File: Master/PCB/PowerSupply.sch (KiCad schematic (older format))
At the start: 32 parts, among them J20 Jumper, Q28 BSS138, Q29 BSS138, Q30 BSS138, U19 LM5165YDRC

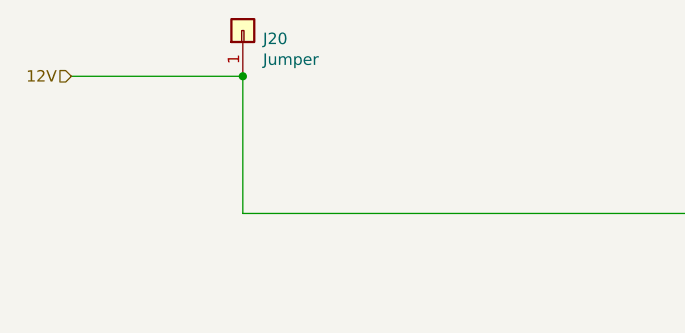
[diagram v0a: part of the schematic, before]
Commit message: Nothing
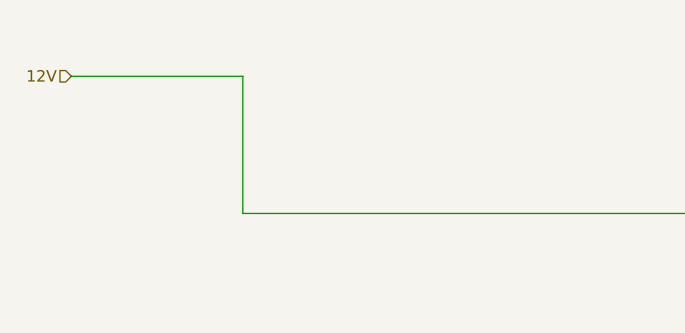
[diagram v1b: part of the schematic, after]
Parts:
- removed J20: Jumper, TestPoint:TestPoint_Loop_D2.54mm_Drill1.5mm_Beaded, symbol BMS-Master-rescue:Conn_01x01-Connector_Generic-BMS-Master-rescue
- R175, R177: footprint Resistors_SMD:R_0805_HandSoldering -> Resistors_SMD:R_0603_HandSoldering
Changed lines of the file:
@@
 $Descr A2 23386 16535
 encoding utf-8
-Sheet 5 7
+Sheet 4 7
 Title ""
 Date ""
@@
 Comment3 ""
 Comment4 ""
-Comment5 ""
-Comment6 ""
-Comment7 ""
-Comment8 ""
-Comment9 ""
 $EndDescr
 Text HLabel 9400 9800 0    50   Input ~ 0
@@
 F 0 "R177" H 13680 6754 50  0000 R CNN
 F 1 "4.7M" H 13680 6845 50  0000 R CNN
-F 2 "Resistors_SMD:R_0805_HandSoldering" V 13680 6800 50  0001 C CNN
+F 2 "Resistors_SMD:R_0603_HandSoldering" V 13680 6800 50  0001 C CNN
 F 3 "~" H 13750 6800 50  0001 C CNN
 	1    13750 6800
@@
 F 0 "R175" H 13280 6754 50  0000 R CNN
 F 1 "4.7M" H 13280 6845 50  0000 R CNN
-F 2 "Resistors_SMD:R_0805_HandSoldering" V 13280 6800 50  0001 C CNN
+F 2 "Resistors_SMD:R_0603_HandSoldering" V 13280 6800 50  0001 C CNN
 F 3 "~" H 13350 6800 50  0001 C CNN
 	1    13350 6800
@@
 Wire Wire Line
 	8650 5800 8650 6400
-Connection ~ 8650 5800
-$Comp
-L BMS-Master-rescue:Conn_01x01-Connector_Generic-BMS-Master-rescue J20
-U 1 1 5C86E7FA
-P 8650 5600
-F 0 "J20" V 8614 5512 50  0000 R CNN
-F 1 "Jumper" V 8523 5512 50  0000 R CNN
-F 2 "TestPoint:TestPoint_Loop_D2.54mm_Drill1.5mm_Beaded" H 8650 5600 50  0001 C CNN
-F 3 "" H 8650 5600 50  0001 C CNN
-	1    8650 5600
-	0    -1   -1   0
-$EndComp
 Wire Wire Line
 	8650 6400 11900 6400
